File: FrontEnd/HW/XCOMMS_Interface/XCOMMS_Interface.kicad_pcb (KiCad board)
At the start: 4 copper layers, 40 x 65 mm, 98 parts, among them J1 TFC-110-02-F-D-A-P-FR, U1 STM32L4, U10 TPS784, U11 AD5160, U12 TPS56637RPAR, U13 MAX870EUK, U14 MAX870EUK, U15 MAX870EUK, U16 TPS56637RPAR, U17 INA290, U9 TPS56637RPAR, Y1 TCXO 10 MHz

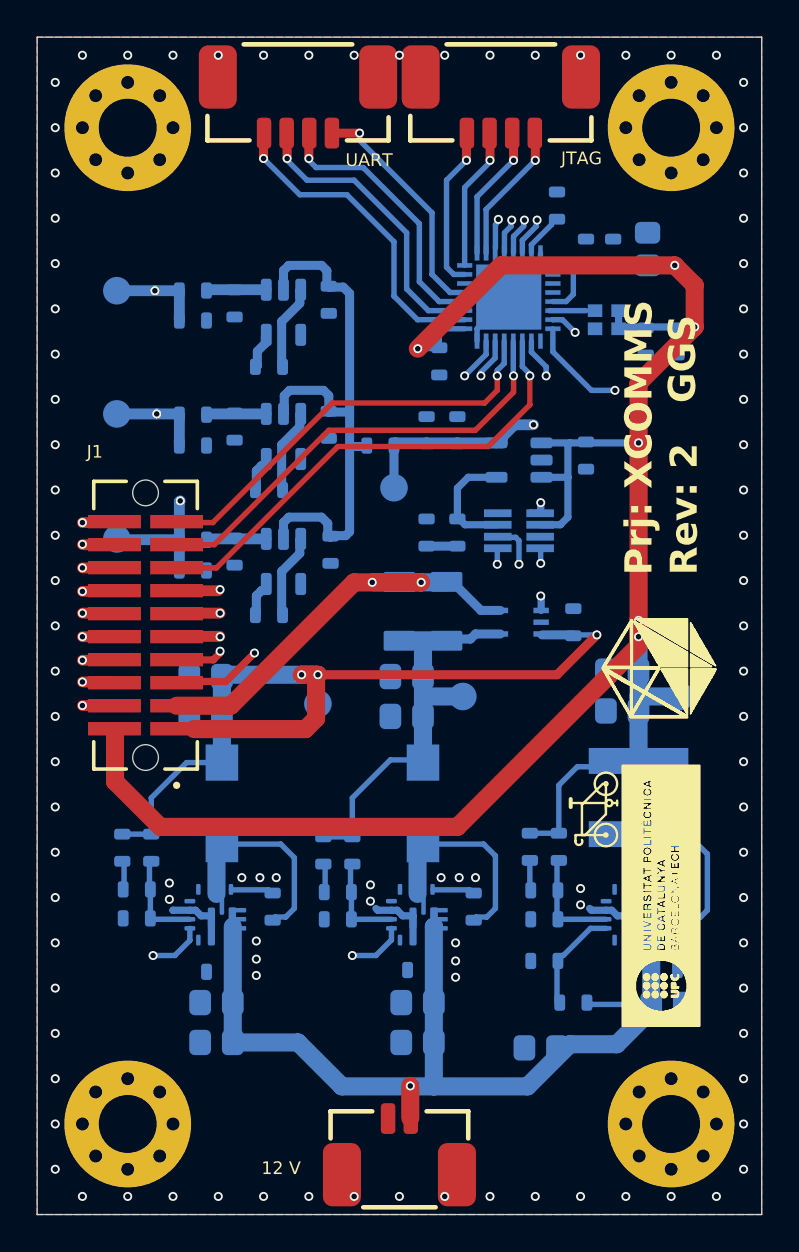
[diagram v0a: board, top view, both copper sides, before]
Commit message: Altium to KiCad translation of interface board
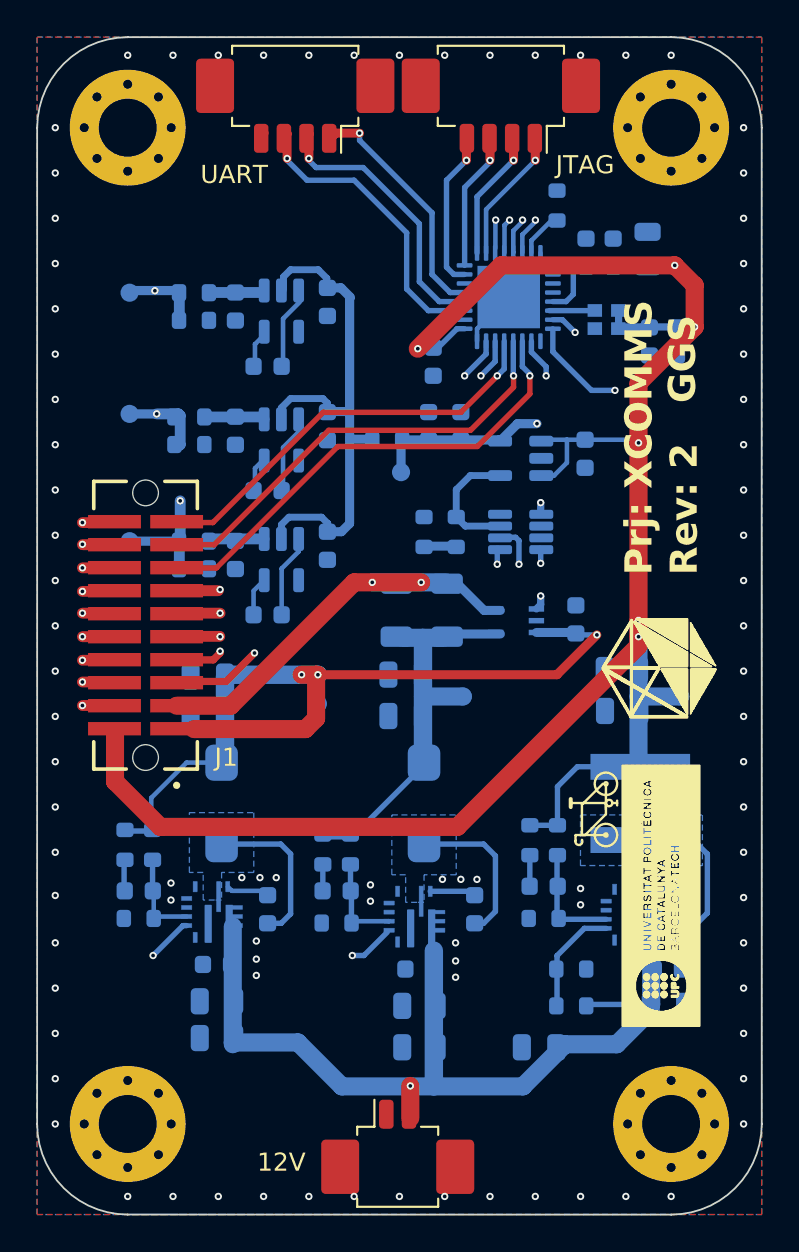
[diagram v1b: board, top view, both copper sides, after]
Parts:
- removed 12 V: MOLEX_52610271, 3CAT_Connectors.PcbLib:532610271
- removed the JTAG at (154.1, 74.7)
- removed the UART at (142.9, 74.7)
- added 12V: MOLEX_52610271, Connector_Molex:Molex_PicoBlade_53261-0271_1x02-1MP_P1.25mm_Horizontal, F.Cu at (148.4, 134.4)
- added Designator10: Comment, D:_GoogleDrive_UPC_MEE_IR_Altium_Library_Altium_libraries_3CAT_Official_lib_3C4_OFFICIAL_LIB.PcbLib_PCB_ID, F.Cu at (144.3, 112.5)
- added JTAG: MOLEX_532610471, Connector_Molex:Molex_PicoBlade_53261-0471_1x04-1MP_P1.25mm_Horizontal, F.Cu at (154.1, 75.7)
- added UART: MOLEX_532610471, Connector_Molex:Molex_PicoBlade_53261-0471_1x04-1MP_P1.25mm_Horizontal, F.Cu at (142.7, 75.7)
- C1: renamed from C2; value Cap Semi -> 4.7uF; footprint Miscellaneous_GGS.PcbLib:0805 SMD Capacitor -> Capacitor_SMD:C_0805_2012Metric
- C10: renamed from C68; value Cap Semi -> 10uF; footprint Miscellaneous_GGS.PcbLib:0805 SMD Capacitor -> Capacitor_SMD:C_0805_2012Metric
- C11: renamed from C69; value Cap Semi -> 10uF; footprint Miscellaneous_GGS.PcbLib:0805 SMD Capacitor -> Capacitor_SMD:C_0805_2012Metric
- C12: renamed from C70; value Cap Semi -> 100nF; footprint Miscellaneous_GGS.PcbLib:0603 SMD Capacitor -> Capacitor_SMD:C_0603_1608Metric
- C13: renamed from C84; value Cap Semi -> 10uF; footprint Miscellaneous_GGS.PcbLib:0805 SMD Capacitor -> Capacitor_SMD:C_0805_2012Metric
- C14: renamed from C85; value Cap Semi -> 10uF; footprint Miscellaneous_GGS.PcbLib:0805 SMD Capacitor -> Capacitor_SMD:C_0805_2012Metric
- C15: renamed from C86; value Cap Semi -> 100nF; footprint Miscellaneous_GGS.PcbLib:0603 SMD Capacitor -> Capacitor_SMD:C_0603_1608Metric
- C16: renamed from C62; value Cap Semi -> 100nF; footprint Miscellaneous_GGS.PcbLib:0603 SMD Capacitor -> Capacitor_SMD:C_0603_1608Metric
- C17: renamed from C77; value Cap Semi -> 100nF; footprint Miscellaneous_GGS.PcbLib:0603 SMD Capacitor -> Capacitor_SMD:C_0603_1608Metric
- C18: renamed from C87; value Cap Semi -> 100nF; footprint Miscellaneous_GGS.PcbLib:0603 SMD Capacitor -> Capacitor_SMD:C_0603_1608Metric
- C19: renamed from C63; value Cap Semi -> 10uF; footprint Miscellaneous_GGS.PcbLib:0805 SMD Capacitor -> Capacitor_SMD:C_0805_2012Metric
- C2: renamed from C1; value Cap Semi -> 1uF; footprint Miscellaneous_GGS.PcbLib:0603 SMD Capacitor -> Capacitor_SMD:C_0603_1608Metric
- C20: renamed from C81; value Cap Semi -> 10uF; footprint Miscellaneous_GGS.PcbLib:0805 SMD Capacitor -> Capacitor_SMD:C_0805_2012Metric
- C21: renamed from C88; value Cap Semi -> 10uF; footprint Miscellaneous_GGS.PcbLib:0805 SMD Capacitor -> Capacitor_SMD:C_0805_2012Metric
- C22: renamed from C67; value Cap Semi -> 10uF; footprint Miscellaneous_GGS.PcbLib:0805 SMD Capacitor -> Capacitor_SMD:C_0805_2012Metric
- C23: renamed from C83; value Cap Semi -> 10uF; footprint Miscellaneous_GGS.PcbLib:0805 SMD Capacitor -> Capacitor_SMD:C_0805_2012Metric
- C24: renamed from C90; value Cap Semi -> 10uF; footprint Miscellaneous_GGS.PcbLib:0805 SMD Capacitor -> Capacitor_SMD:C_0805_2012Metric
- C25: renamed from C64; value Cap Semi -> 100pF; footprint Miscellaneous_GGS.PcbLib:0603 SMD Capacitor -> Capacitor_SMD:C_0603_1608Metric
- C26: renamed from C82; value Cap Semi -> 100pF; footprint Miscellaneous_GGS.PcbLib:0603 SMD Capacitor -> Capacitor_SMD:C_0603_1608Metric
- C27: renamed from C89; value Cap Semi -> 100pF; footprint Miscellaneous_GGS.PcbLib:0603 SMD Capacitor -> Capacitor_SMD:C_0603_1608Metric
- C28: renamed from C7; value Cap Semi -> 100nF; footprint Miscellaneous_GGS.PcbLib:0603 SMD Capacitor -> Capacitor_SMD:C_0603_1608Metric
- C29: renamed from C78; value Cap Semi -> 0.33uF; footprint Miscellaneous_GGS.PcbLib:0603 SMD Capacitor -> Capacitor_SMD:C_0603_1608Metric
- C3, C4, C6: value Cap Semi -> 100nF; footprint Miscellaneous_GGS.PcbLib:0603 SMD Capacitor -> Capacitor_SMD:C_0603_1608Metric
- C30: renamed from C61; value Cap Semi -> 1uF; footprint Miscellaneous_GGS.PcbLib:0603 SMD Capacitor -> Capacitor_SMD:C_0603_1608Metric
- C31: renamed from C65; value Cap Semi -> 1uF; footprint Miscellaneous_GGS.PcbLib:0603 SMD Capacitor -> Capacitor_SMD:C_0603_1608Metric
- C32: renamed from C66; value Cap Semi -> 1uF; footprint Miscellaneous_GGS.PcbLib:0603 SMD Capacitor -> Capacitor_SMD:C_0603_1608Metric
- C33: renamed from C71; value Cap Semi -> 0.33uF; footprint Miscellaneous_GGS.PcbLib:0603 SMD Capacitor -> Capacitor_SMD:C_0603_1608Metric
- C34: renamed from C74; value Cap Semi -> 0.33uF; footprint Miscellaneous_GGS.PcbLib:0603 SMD Capacitor -> Capacitor_SMD:C_0603_1608Metric
- C35: renamed from C79; value Cap Semi -> 0.33uF; footprint Miscellaneous_GGS.PcbLib:0603 SMD Capacitor -> Capacitor_SMD:C_0603_1608Metric
- C36: renamed from C72; value Cap Semi -> 0.33uF; footprint Miscellaneous_GGS.PcbLib:0603 SMD Capacitor -> Capacitor_SMD:C_0603_1608Metric
- C37: renamed from C75; value Cap Semi -> 0.33uF; footprint Miscellaneous_GGS.PcbLib:0603 SMD Capacitor -> Capacitor_SMD:C_0603_1608Metric
- C38: renamed from C80; value Cap Semi -> 0.33uF; footprint Miscellaneous_GGS.PcbLib:0603 SMD Capacitor -> Capacitor_SMD:C_0603_1608Metric
- C39: renamed from C73; value Cap Semi -> 0.33uF; footprint Miscellaneous_GGS.PcbLib:0603 SMD Capacitor -> Capacitor_SMD:C_0603_1608Metric
- C40: renamed from C76; value Cap Semi -> 0.33uF; footprint Miscellaneous_GGS.PcbLib:0603 SMD Capacitor -> Capacitor_SMD:C_0603_1608Metric
- C5: value Cap Semi -> 1uF; footprint Miscellaneous_GGS.PcbLib:0603 SMD Capacitor -> Capacitor_SMD:C_0603_1608Metric
- C7: renamed from C58; value Cap Semi -> 10uF; footprint Miscellaneous_GGS.PcbLib:0805 SMD Capacitor -> Capacitor_SMD:C_0805_2012Metric
- C8: renamed from C59; value Cap Semi -> 10uF; footprint Miscellaneous_GGS.PcbLib:0805 SMD Capacitor -> Capacitor_SMD:C_0805_2012Metric
- C9: renamed from C60; value Cap Semi -> 100nF; footprint Miscellaneous_GGS.PcbLib:0603 SMD Capacitor -> Capacitor_SMD:C_0603_1608Metric
- J1: footprint Connectors_GGS.PcbLib:SAMTEC_TFC-110-02-F-D-A-P-FR -> GGS_Connectors:SAMTEC_TFC-110-02-F-D-A-P-FR
- L1: renamed from L3; value 652-SRP5030T-3R3M -> 3.3uH; footprint Miscellaneous_GGS.PcbLib:Bourns_SRP5030T-3R3M -> Inductor_SMD:L_Bourns_SRP5030T
- L2: renamed from L4; value 652-SRP5030T-3R3M -> 3.3uH; footprint Miscellaneous_GGS.PcbLib:Bourns_SRP5030T-3R3M -> Inductor_SMD:L_Bourns_SRP5030T
- L3: renamed from L5; value WE_74438356022 -> 2.2uH; footprint Miscellaneous_GGS.PcbLib:Coilcraft_XAL60xx -> Inductor_SMD:L_Coilcraft_XAL60xx_6.36x6.56mm
- R1: value Res3 -> 510; footprint Miscellaneous_GGS.PcbLib:0603 SMD Resistor -> Resistor_SMD:R_0603_1608Metric
- R10: renamed from R12; value Res3 -> 10k; footprint Miscellaneous_GGS.PcbLib:0603 SMD Resistor -> Resistor_SMD:R_0603_1608Metric
- R11: renamed from R18; value Res3 -> 10k; footprint Miscellaneous_GGS.PcbLib:0603 SMD Resistor -> Resistor_SMD:R_0603_1608Metric
- R12: renamed from R29; value Res3 -> 10k; footprint Miscellaneous_GGS.PcbLib:0603 SMD Resistor -> Resistor_SMD:R_0603_1608Metric
- R13: renamed from R19; value Res3 -> 10k; footprint Miscellaneous_GGS.PcbLib:0603 SMD Resistor -> Resistor_SMD:R_0603_1608Metric
- R14: renamed from R17; value Res3 -> 0R; footprint Miscellaneous_GGS.PcbLib:0603 SMD Resistor -> Resistor_SMD:R_0603_1608Metric
- R15: renamed from R24; value Res3 -> 20k; footprint Miscellaneous_GGS.PcbLib:0603 SMD Resistor -> Resistor_SMD:R_0603_1608Metric
- R16: renamed from R20; value Res3 -> 10k; footprint Miscellaneous_GGS.PcbLib:0603 SMD Resistor -> Resistor_SMD:R_0603_1608Metric
- R17: renamed from R25; value Res3 -> 20k; footprint Miscellaneous_GGS.PcbLib:0603 SMD Resistor -> Resistor_SMD:R_0603_1608Metric
- R18: renamed from R14; value Res3 -> 20k; footprint Miscellaneous_GGS.PcbLib:0603 SMD Resistor -> Resistor_SMD:R_0603_1608Metric
- R19: renamed from R15; value Res3 -> 5k; footprint Miscellaneous_GGS.PcbLib:0603 SMD Resistor -> Resistor_SMD:R_0603_1608Metric
- R2: renamed from R27; value Res3 -> 169k; footprint Miscellaneous_GGS.PcbLib:0603 SMD Resistor -> Resistor_SMD:R_0603_1608Metric
- R20: renamed from R21; value Res3 -> 10k; footprint Miscellaneous_GGS.PcbLib:0603 SMD Resistor -> Resistor_SMD:R_0603_1608Metric
- R21: renamed from R26; value Res3 -> 20k; footprint Miscellaneous_GGS.PcbLib:0603 SMD Resistor -> Resistor_SMD:R_0603_1608Metric
- R3: renamed from R13; value Res3 -> 90.9k; footprint Miscellaneous_GGS.PcbLib:0603 SMD Resistor -> Resistor_SMD:R_0603_1608Metric
- R4: renamed from R16; value Res3 -> 20k; footprint Miscellaneous_GGS.PcbLib:0603 SMD Resistor -> Resistor_SMD:R_0603_1608Metric
- R5: renamed from R22; value Res3 -> 73.2k; footprint Miscellaneous_GGS.PcbLib:0603 SMD Resistor -> Resistor_SMD:R_0603_1608Metric
- R6: renamed from R23; value Res3 -> 20k; footprint Miscellaneous_GGS.PcbLib:0603 SMD Resistor -> Resistor_SMD:R_0603_1608Metric
- R7: renamed from R30; value Res3 -> 45.3k; footprint Miscellaneous_GGS.PcbLib:0603 SMD Resistor -> Resistor_SMD:R_0603_1608Metric
- R8: renamed from R31; value Res3 -> 20k; footprint Miscellaneous_GGS.PcbLib:0603 SMD Resistor -> Resistor_SMD:R_0603_1608Metric
- R9: renamed from R28; value Res3 -> 36.1k; footprint Miscellaneous_GGS.PcbLib:0603 SMD Resistor -> Resistor_SMD:R_0603_1608Metric
- Rsense1, Rsense2: value Res3 -> 0R005; footprint Miscellaneous_GGS.PcbLib:1206 SMD RESISTOR -> Resistor_SMD:R_1206_3216Metric
- SCRW1, SCRW2, SCRW3, SCRW4: value Metric Screw Hole -> MountingHole_Pad; footprint 3CAT_Miscellaneous.PcbLib:M3 ScrewHole -> MountingHole:MountingHole_3.2mm_M3_Pad_Via
- TP1: renamed from TP4; value TP -> TestPoint; footprint Connectors_GGS.PcbLib:TestPoint -> TestPoint:TestPoint_Pad_D1.0mm
- TP2: renamed from TP6; value TP -> TestPoint; footprint Connectors_GGS.PcbLib:TestPoint -> TestPoint:TestPoint_Pad_D1.0mm
- TP3: renamed from TP10; value TP -> TestPoint; footprint Connectors_GGS.PcbLib:TestPoint -> TestPoint:TestPoint_Pad_D1.0mm
- TP4: renamed from TP7; value TP -> TestPoint; footprint Connectors_GGS.PcbLib:TestPoint -> TestPoint:TestPoint_Pad_D1.0mm
- TP5: value TP -> TestPoint; footprint Connectors_GGS.PcbLib:TestPoint -> TestPoint:TestPoint_Pad_D1.0mm
- TP6: renamed from TP8; value TP -> TestPoint; footprint Connectors_GGS.PcbLib:TestPoint -> TestPoint:TestPoint_Pad_D1.0mm
- TP7: renamed from TP9; value TP -> TestPoint; footprint Connectors_GGS.PcbLib:TestPoint -> TestPoint:TestPoint_Pad_D1.0mm
- U1: value STM32L4 -> STM32L431KBUx; footprint Miscellaneous_GGS.PcbLib:QFN-33N -> Package_DFN_QFN:QFN-32-1EP_5x5mm_P0.5mm_EP3.45x3.45mm
- U10: renamed from U15; footprint Power_GGS.PcbLib:SOT23-5N -> Package_TO_SOT_SMD:SOT-23-5
- U2: renamed from U9; value TPS56637RPAR -> TPS56637; footprint Power_GGS.PcbLib:CONV_TPS56637RPAR -> GGS_Power:TPS56637RPAR
- U3: renamed from U12; value TPS56637RPAR -> TPS56637; footprint Power_GGS.PcbLib:CONV_TPS56637RPAR -> GGS_Power:TPS56637RPAR
- U4: renamed from U16; value TPS56637RPAR -> TPS56637; footprint Power_GGS.PcbLib:CONV_TPS56637RPAR -> GGS_Power:TPS56637RPAR
- U5: renamed from U10; footprint Power_GGS.PcbLib:SOT23-5N -> Package_TO_SOT_SMD:SOT-23-5
- U6: renamed from U13; footprint Power_GGS.PcbLib:SOT23-5N -> Package_TO_SOT_SMD:SOT-23-5
- U7: renamed from U17; footprint Miscellaneous_GGS.PcbLib:SC70-5 -> GGS_Miscellaneous:SC70-5
- U8: renamed from U11; footprint Miscellaneous_GGS.PcbLib:SOT-28-8N -> Package_TO_SOT_SMD:SOT-23-8
- U9: renamed from U14; footprint Power_GGS.PcbLib:SOT23-5N -> Package_TO_SOT_SMD:SOT-23-5
- Y1: value TCXO 10 MHz -> TCXO_ECS; footprint Miscellaneous_GGS.PcbLib:ECS-TXO-2016 -> GGS_Miscellaneous:TCXO_ECS
- moved U3 5.25 mm to (138.7, 115.7)
- moved U4 5.12 mm to (161.9, 115.9)
- moved Y1 5.07 mm to (160.6, 92.7)
- moved U7 5.00 mm to (154.9, 109.8)
- moved U2 5.00 mm to (149.9, 116.0)
- moved R9 1.55 mm to (158.0, 124.0), turned to 0 degrees
- moved TP5 0.94 mm to (148.6, 96.5)
- moved TP7 0.71 mm to (133.6, 100.3)
- moved TP4 0.71 mm to (133.6, 86.6)
- moved TP6 0.70 mm to (133.6, 93.3)
- moved R14 0.49 mm to (147.8, 94.7)
- moved C12 0.44 mm to (138.4, 123.7)
- moved R7 0.37 mm to (157.2, 116.8)
- moved R8 0.36 mm to (155.7, 116.8), turned to -90 degrees
- moved L3 0.34 mm to (161.8, 114.8)
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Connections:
- net 5V_EN renamed /5V_EN
- net 6V_EN renamed /6V_EN
- net CurrentSense renamed /CurrentSense
- net LO_EN renamed /LO_EN
- net NetC65_1 renamed Net-(C31-Pad1)
- net NetR27_2 renamed Net-(R2-Pad2)
- net PLL_CSB renamed /PLL_CSB
- net R_CSB renamed /R_CSB
- net SCK renamed /SCK
- net SDI renamed /SDI
- net SDO renamed /SDO
- net T_CSB renamed /T_CSB
- net Tx_CE renamed /Tx_CE
- net Tx_PM renamed /Tx_PM
- net Vd_PA renamed /Vd_PA
- net mcu_OSC renamed /mcu_OSC
- C1 pad 1: GND -> +3V3
- C1 pad 2: 3V3 -> GND
- C10 pad 1: GND -> +12V
- C10 pad 2: 12V -> GND
- C11 pad 1: GND -> +12V
- C11 pad 2: 12V -> GND
- C12 pad 1: 12V -> +12V
- C13 pad 1: GND -> +12V
- C13 pad 2: 12V -> GND
- C14 pad 1: GND -> +12V
- C14 pad 2: 12V -> GND
- C15 pad 1: 12V -> +12V
- C16 pad 1: NetC62_1 -> Net-(C16-Pad1)
- C16 pad 2: NetC62_2 -> Net-(C16-Pad2)
- C17 pad 1: NetC77_1 -> Net-(C17-Pad1)
- C17 pad 2: NetC77_2 -> Net-(C17-Pad2)
- C18 pad 1: NetC87_1 -> Net-(C18-Pad1)
- C18 pad 2: NetC87_2 -> Net-(C18-Pad2)
- C19 pad 1: GND -> /XCOMMS_PowerSupply/6V
- C19 pad 2: 6V -> GND
- C2 pad 1: GND -> +3V3
- C2 pad 2: 3V3 -> GND
- C20 pad 1: GND -> +5V
- C20 pad 2: 5V -> GND
- C21 pad 1: GND -> +3V3
- C21 pad 2: 3V3 -> GND
- C22 pad 1: GND -> /XCOMMS_PowerSupply/6V
- C22 pad 2: 6V -> GND
- C23 pad 1: GND -> +5V
- C23 pad 2: 5V -> GND
- C24 pad 1: GND -> +3V3
- C24 pad 2: 3V3 -> GND
- C25 pad 1: NetC64_1 -> Net-(C25-Pad1)
- C25 pad 2: NetC64_2 -> Net-(C25-Pad2)
- C26 pad 1: NetC82_1 -> Net-(C26-Pad1)
- C26 pad 2: NetC82_2 -> Net-(C26-Pad2)
- C27 pad 1: NetC89_1 -> Net-(C27-Pad1)
- C27 pad 2: NetC89_2 -> Net-(C27-Pad2)
- C28 pad 1: 5V -> GND
- C28 pad 2: GND -> +5V
- C29 pad 1: NetC78_1 -> GND
- C29 pad 2: GND -> Net-(C29-Pad2)
- C3 pad 1: 3V3 -> +3V3
- C30 pad 1: 3V3 -> +3V3
- C33 pad 1: Vinv_in -> GND
- C33 pad 2: GND -> /XCOMMS_PowerSupply/Vinv_in
- C34 pad 1: NetC74_1 -> Net-(C34-Pad1)
- C34 pad 2: NetC74_2 -> Net-(C34-Pad2)
- C35 pad 1: NetC79_1 -> GND
- C35 pad 2: GND -> Net-(C35-Pad2)
- C36 pad 1: Vinv_in -> GND
- C36 pad 2: GND -> /XCOMMS_PowerSupply/Vinv_in
- C37 pad 1: NetC75_1 -> Net-(C37-Pad1)
- C37 pad 2: NetC75_2 -> Net-(C37-Pad2)
- C38 pad 1: NetC80_1 -> GND
- C38 pad 2: GND -> Net-(C38-Pad2)
- C39 pad 1: Vinv_in -> GND
- C39 pad 2: GND -> /XCOMMS_PowerSupply/Vinv_in
- C4 pad 1: 3V3 -> +3V3
- C40 pad 1: NetC76_1 -> Net-(C40-Pad1)
- C40 pad 2: NetC76_2 -> Net-(C40-Pad2)
- C5 pad 1: GND -> +3V3
- C5 pad 2: 3V3 -> GND
- C6 pad 1: 3V3 -> +3V3
- C7 pad 1: GND -> +12V
- C7 pad 2: 12V -> GND
- C8 pad 1: GND -> +12V
- C8 pad 2: 12V -> GND
- C9 pad 1: 12V -> +12V
- J1 pad 01: 5V -> +5V
- J1 pad 02: 3V3 -> +3V3
- J1 pad 16: Vg_PA3 -> /Vg_PA3
- J1 pad 18: Vg_PA2 -> /Vg_PA2
- J1 pad 20: Vg_PA1 -> /Vg_PA1
- L1 pad 1: NetC62_1 -> Net-(C16-Pad2)
- L1 pad 2: 6V -> /XCOMMS_PowerSupply/6V
- L2 pad 1: NetC77_1 -> Net-(C17-Pad2)
- L2 pad 2: 5V -> +5V
- L3 pad 1: NetC87_1 -> Net-(C18-Pad2)
- L3 pad 2: 3V3 -> +3V3
- R1 pad 1: GND -> /Boot0
- R1 pad 2: NetR1_2 -> GND
- R10 pad 1: NetC64_2 -> Net-(C25-Pad1)
- R11 pad 1: NetC82_2 -> Net-(C26-Pad1)
- R12 pad 1: NetC89_2 -> Net-(C27-Pad1)
- R13 pad 1: NetC78_1 -> Net-(C29-Pad2)
- R13 pad 2: Vg_PA1 -> /Vg_PA1
- R14 pad 2: Vinv_in -> /XCOMMS_PowerSupply/Vinv_in
- R15 pad 1: GND -> /Vg_PA1
- R15 pad 2: Vg_PA1 -> GND
- R16 pad 1: NetC79_1 -> Net-(C35-Pad2)
- R16 pad 2: Vg_PA2 -> /Vg_PA2
- R17 pad 1: GND -> /Vg_PA2
- R17 pad 2: Vg_PA2 -> GND
- R18 pad 1: NetR14_1 -> Net-(R18-Pad1)
- R18 pad 2: NetR14_2 -> Net-(R18-Pad2)
- R19 pad 1: GND -> Net-(R18-Pad2)
- R19 pad 2: NetR14_1 -> GND
- R2 pad 1: 12V -> +12V
- R20 pad 1: NetC80_1 -> Net-(C38-Pad2)
- R20 pad 2: Vg_PA3 -> /Vg_PA3
- R21 pad 1: GND -> /Vg_PA3
- R21 pad 2: Vg_PA3 -> GND
- R3 pad 1: NetC64_2 -> /XCOMMS_PowerSupply/6V
- R3 pad 2: 6V -> Net-(C25-Pad1)
- R4 pad 1: NetC64_1 -> /XCOMMS_PowerSupply/6V
- R4 pad 2: 6V -> Net-(C25-Pad2)
- R5 pad 1: 5V -> +5V
- R5 pad 2: NetC82_2 -> Net-(C26-Pad1)
- R6 pad 1: NetC82_1 -> +5V
- R6 pad 2: 5V -> Net-(C26-Pad2)
- R7 pad 1: 3V3 -> +3V3
- R7 pad 2: NetC89_2 -> Net-(C27-Pad1)
- R8 pad 1: NetC89_1 -> +3V3
- R8 pad 2: 3V3 -> Net-(C27-Pad2)
- Rsense1 pad 1: 6V -> /XCOMMS_PowerSupply/6V
- Rsense2 pad 1: 6V -> /XCOMMS_PowerSupply/6V
- TP1 pad 1: 6V -> /XCOMMS_PowerSupply/6V
- TP2 pad 1: 5V -> +5V
- TP3 pad 1: 3V3 -> +3V3
- TP4 pad 1: Vg_PA1 -> /Vg_PA1
- TP6 pad 1: Vg_PA2 -> /Vg_PA2
- TP7 pad 1: Vg_PA3 -> /Vg_PA3
- U1 pad 1: 3V3 -> +3V3
- U1 pad 17: 3V3 -> +3V3
- U1 pad 18: USART1_CK -> unconnected-(U1-Pad18)
- U1 pad 19: USART1_Tx -> /USART1_Tx
- U1 pad 2: (no net) -> unconnected-(U1-Pad2)
- U1 pad 20: USART1_Rx -> /USART1_Rx
- U1 pad 21: USART1_CTS -> /USART1_CTS
- U1 pad 22: (no net) -> unconnected-(U1-Pad22)
- U1 pad 23: JTMS -> /JTMS
- U1 pad 24: JTCK -> /JTCK
- U1 pad 25: JTDI -> /JTDI
- U1 pad 26: JTDO -> /JTDO
- U1 pad 3: (no net) -> unconnected-(U1-Pad3)
- U1 pad 31: NetR1_2 -> /Boot0
- U1 pad 4: (no net) -> unconnected-(U1-Pad4)
- U1 pad 5: 3V3 -> +3V3
- U1 pad 9: (no net) -> unconnected-(U1-Pad9)
- U10 pad 1: NetC80_1 -> Net-(C38-Pad2)
- U10 pad 2: Vinv_in -> /XCOMMS_PowerSupply/Vinv_in
- U10 pad 3: NetC76_2 -> Net-(C40-Pad1)
- U10 pad 5: NetC76_1 -> Net-(C40-Pad2)
- U2 pad 2: NetC64_2 -> Net-(C25-Pad1)
- U2 pad 4: (no net) -> unconnected-(U2-Pad4)
- U2 pad 5: (no net) -> unconnected-(U2-Pad5)
- U2 pad 6: NetC62_1 -> Net-(C16-Pad2)
- U2 pad 7: NetC62_2 -> Net-(C16-Pad1)
- U2 pad 8: 12V -> +12V
- U3 pad 2: NetC82_2 -> Net-(C26-Pad1)
- U3 pad 4: (no net) -> unconnected-(U3-Pad4)
- U3 pad 5: (no net) -> unconnected-(U3-Pad5)
- U3 pad 6: NetC77_1 -> Net-(C17-Pad2)
- U3 pad 7: NetC77_2 -> Net-(C17-Pad1)
- U3 pad 8: 12V -> +12V
- U4 pad 2: NetC89_2 -> Net-(C27-Pad1)
- U4 pad 4: (no net) -> unconnected-(U4-Pad4)
- U4 pad 5: (no net) -> unconnected-(U4-Pad5)
- U4 pad 6: NetC87_1 -> Net-(C18-Pad2)
- U4 pad 7: NetC87_2 -> Net-(C18-Pad1)
- U4 pad 8: 12V -> +12V
- U5 pad 1: 3V3 -> +3V3
- U5 pad 3: 3V3 -> +3V3
- U5 pad 4: NetR14_2 -> Net-(R18-Pad1)
- U6 pad 1: NetC78_1 -> Net-(C29-Pad2)
- U6 pad 2: Vinv_in -> /XCOMMS_PowerSupply/Vinv_in
- U6 pad 3: NetC74_2 -> Net-(C34-Pad1)
- U6 pad 5: NetC74_1 -> Net-(C34-Pad2)
- U7 pad 3: 5V -> +5V
- U7 pad 4: 6V -> /XCOMMS_PowerSupply/6V
- U8 pad 2: 3V3 -> unconnected-(U8-Pad2)
- U8 pad 7: NetR14_2 -> Net-(R18-Pad1)
- U8 pad 8: (no net) -> unconnected-(U8-Pad8)
- U9 pad 1: NetC79_1 -> Net-(C35-Pad2)
- U9 pad 2: Vinv_in -> /XCOMMS_PowerSupply/Vinv_in
- U9 pad 3: NetC75_2 -> Net-(C37-Pad1)
- U9 pad 5: NetC75_1 -> Net-(C37-Pad2)
- Y1 pad 1: 3V3 -> +3V3
- Y1 pad 4: 3V3 -> +3V3
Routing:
- net 3V3: track 126.9 -> 0.00 mm, vias 6 -> 0
- net +3V3: track 0.00 -> 121.9 mm, vias 0 -> 6
- net 12V: track 50.6 -> 0.00 mm, vias 1 -> 0
- net 5V: track 50.2 -> 0.00 mm, vias 3 -> 0
- net +12V: track 0.00 -> 49.8 mm, vias 0 -> 1
- net +5V: track 0.00 -> 49.6 mm, vias 0 -> 3
- net Vinv_in: track 31.5 -> 0.00 mm
- net /XCOMMS_PowerSupply/Vinv_in: track 0.00 -> 29.6 mm
- net 6V: track 22.7 -> 0.00 mm
- net Vg_PA1: track 22.3 -> 0.00 mm, vias 2 -> 0
- net /Vg_PA1: track 0.00 -> 21.6 mm, vias 0 -> 2
- net /XCOMMS_PowerSupply/6V: track 0.00 -> 21.5 mm
- net USART1_CK: track 18.0 -> 0.00 mm, vias 1 -> 0
- net Vg_PA2: track 17.0 -> 0.00 mm, vias 2 -> 0
- net USART1_Tx: track 16.5 -> 0.00 mm, vias 1 -> 0
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- added copper zone on B.Cu, net Net-(C16-Pad2)
- added copper zone on B.Cu, net Net-(C17-Pad2)
- added copper zone on B.Cu, net Net-(C18-Pad2)
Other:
- outline, holes or cut-outs redrawn
